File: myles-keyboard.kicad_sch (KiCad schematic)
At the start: 52 parts, among them J1 TRRS, J2 OLED, SW01 Key, SW02 Key, SW03 Key, SW04 Key, SW11 Key, SW12 Key, SW13 Key, SW14 Key, SW15 Key, SW16 Key, SW17 Key, SW18 Key, SW19 Key, SW21 Key, SW22 Key, SW23 Key, SW24 Key, SW25 Key, SW26 Key, SW27 Key, SW28 Key, SW29 Key, SW30 Key, SW31 Key, SW32 Key, SW33 Key, SW34 Key, SW35 Key, SW36 Key, SW37 Key, SW38 Key, SW39 Key, SW40 Key, SW41 Key, SW42 Key, SW43 Key, SW44 Key, SW45 Key, SW46 Key, SW47 Key, SW48 Key, SW49 Key, U1 ProMicro

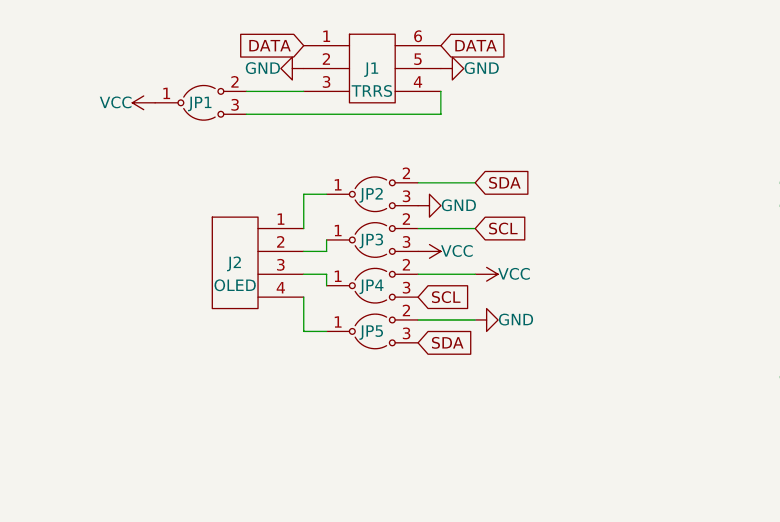
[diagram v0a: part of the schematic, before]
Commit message: reorder jumpers
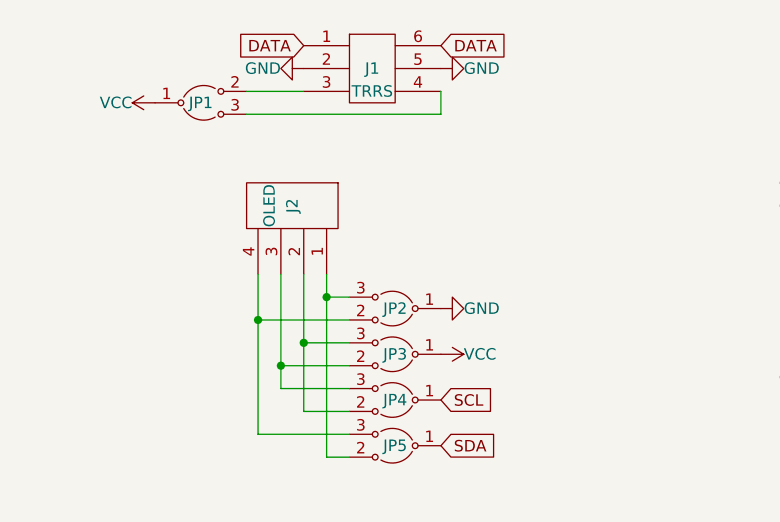
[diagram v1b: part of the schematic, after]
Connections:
- net GND: now also JP2.1; no longer JP2.3, JP5.2
- net SCL: now also JP4.1; no longer JP3.2, JP4.3
- net SDA: now also JP5.1; no longer JP2.2, JP5.3
- net VCC: now also JP3.1; no longer JP3.3, JP4.2
- net at J2.1: now also JP2.3, JP5.2; no longer JP2.1
- net at J2.2: now also JP3.3, JP4.2; no longer JP3.1
- net at J2.3: now also JP3.2, JP4.3; no longer JP4.1
- net at J2.4: now also JP2.2, JP5.3; no longer JP5.1
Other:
- moved on the sheet: J2, JP2, JP3, JP4, JP5
